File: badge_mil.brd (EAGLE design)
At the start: 77.2 x 83.1 mm, 29 parts, among them U1 TINY2313-*S*, X1 FH12-10S-0.5S

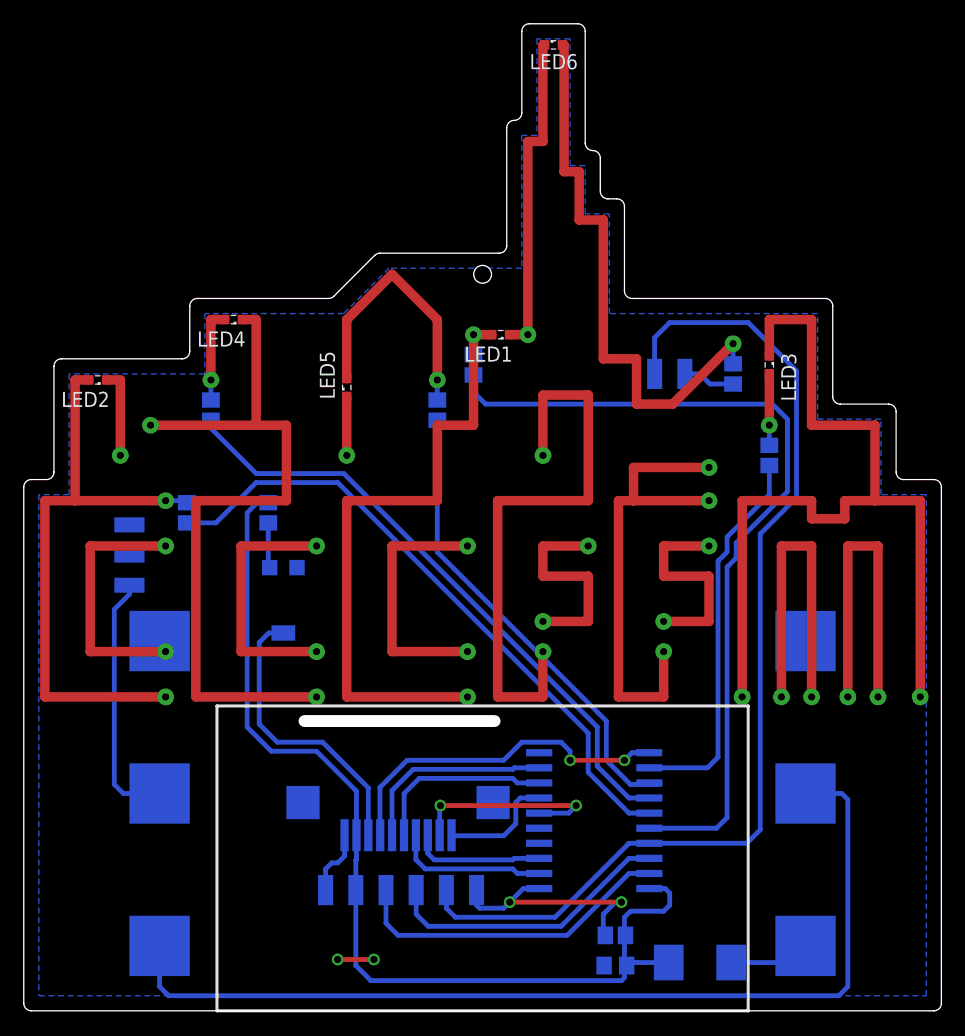
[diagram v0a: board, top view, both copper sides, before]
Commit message: minor tweaks
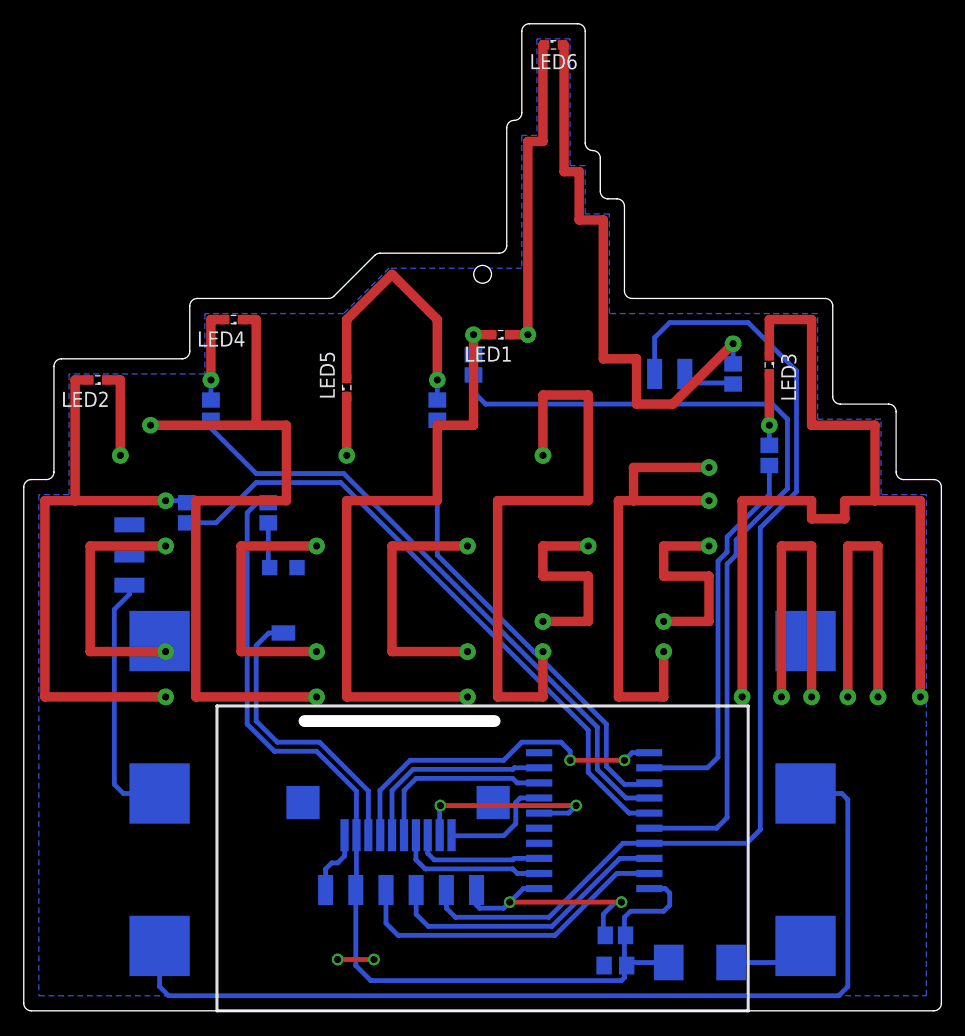
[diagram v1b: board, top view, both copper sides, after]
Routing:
- net N$13: track 90.6 -> 91.3 mm
